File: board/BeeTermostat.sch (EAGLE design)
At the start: 32 parts, among them IC1 7805T, IC2 LD1117S33, K1 TRIL-5VDC, Q1 BC546A, X5 DS18B20

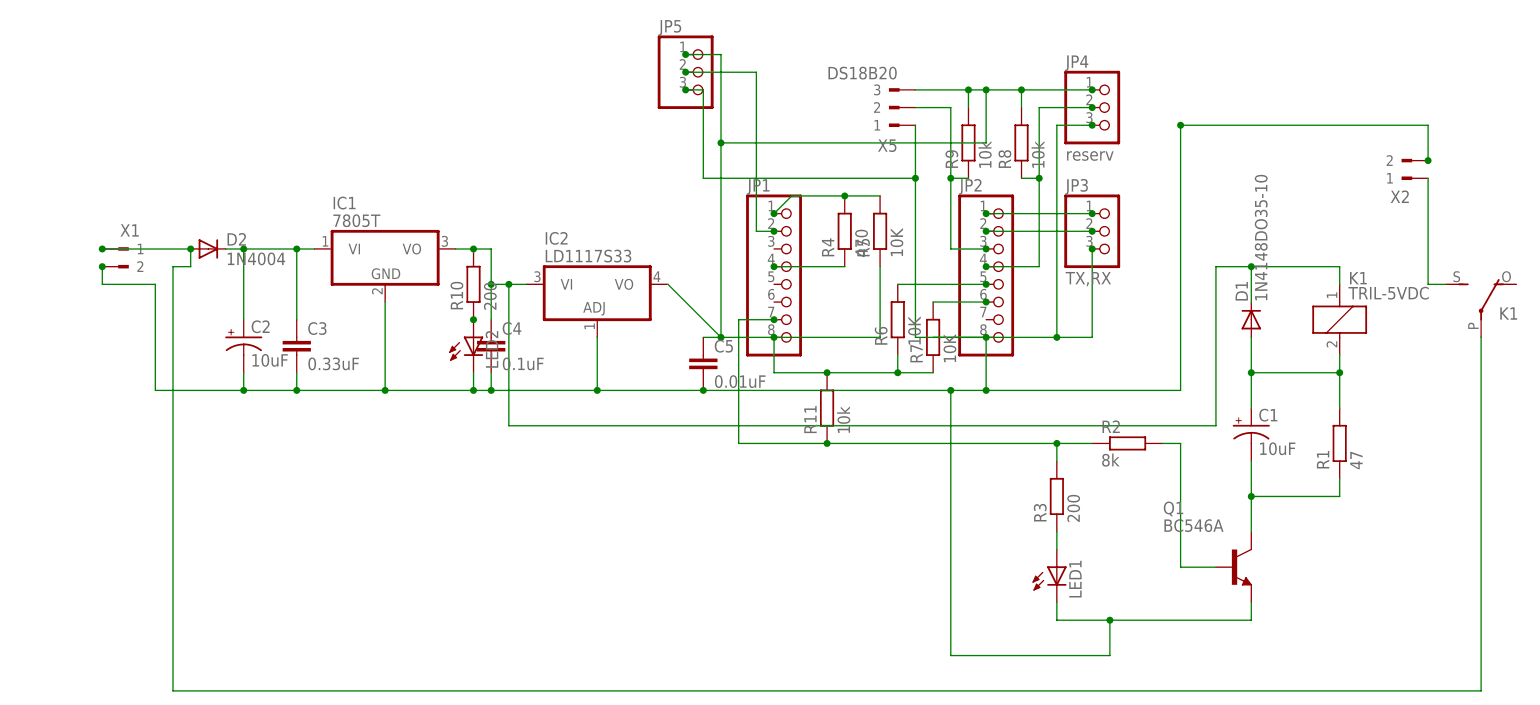
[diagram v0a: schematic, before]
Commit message: update
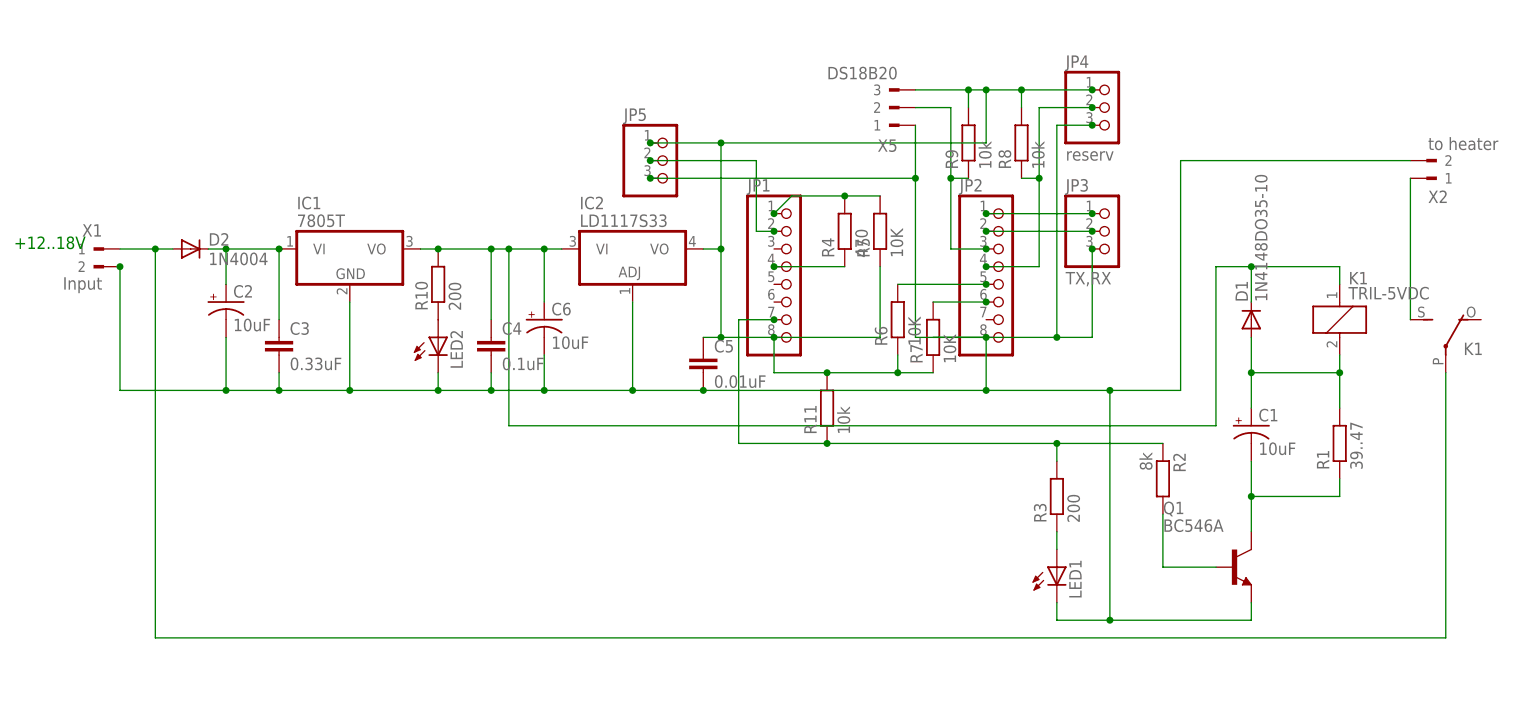
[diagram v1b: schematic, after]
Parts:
- added C6: 10uF, rcl:CPOL-USE5-8.5
- R1: value 47 -> 39..47
- X1: value (none) -> Input
- X2: value (none) -> to heater
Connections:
- removed net N$14: C2.-, C3.2, C4.2, C5.2, IC1.GND, IC2.ADJ, JP2.8, JP3.3, JP4.3, JP5.3, LED1.C, LED2.C, Q1.E, X1.2, X2.2, X5.1
- new net N$42: C2.-, C3.2, C4.2, C5.2, C6.-, IC1.GND, IC2.ADJ, JP2.8, JP3.3, JP4.3, JP5.3, LED1.C, LED2.C, Q1.E, X1.2, X2.2, X5.1
- net N$9: now also C6.+
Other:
- note added: "+12..18V"
- moved on the sheet: C2, C3, D2, IC1, IC2, JP5, K1, LED2, R10, R2, X1, X2
